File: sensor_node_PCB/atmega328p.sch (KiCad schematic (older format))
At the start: 14 parts, among them SW1 RESET_SWITCH, U5 ATMEGA328P, X2 CSTCE16MOV53-R0

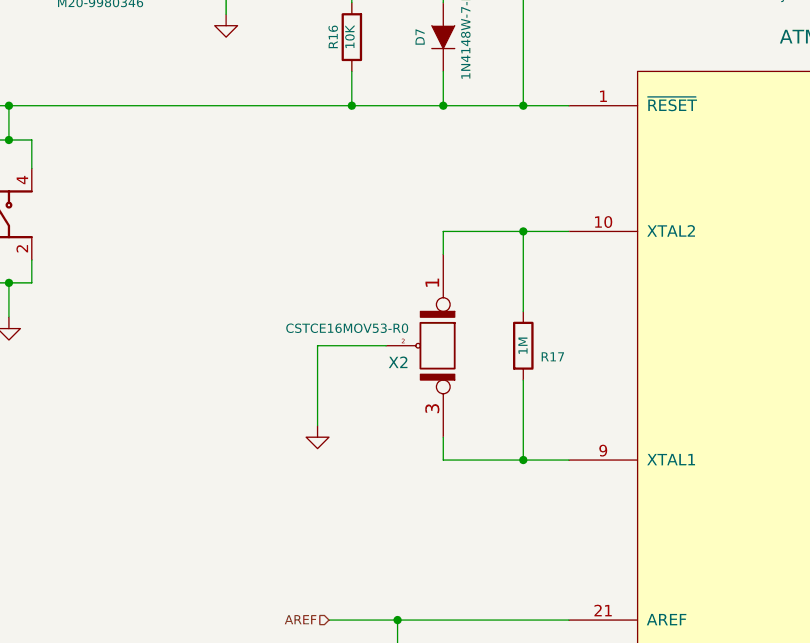
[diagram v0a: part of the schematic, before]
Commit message: routing started 15%
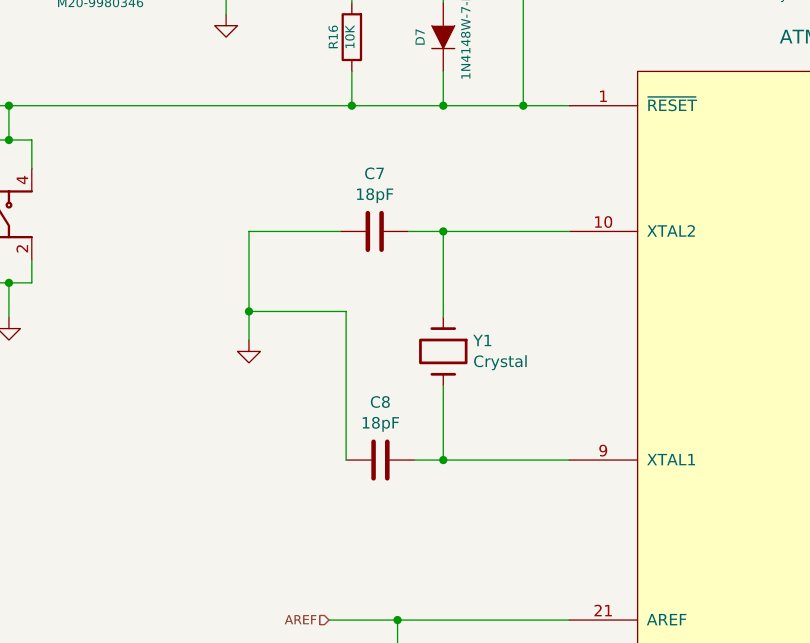
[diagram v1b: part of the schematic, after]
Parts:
- removed R17: 1M, Resistor_SMD:R_0603_1608Metric, symbol Arduino_Uno_R3_From_Scratch-rescue:R
- removed X2: CSTCE16MOV53-R0, symbol Arduino_Uno_R3_From_Scratch-rescue:CERAMIC_RESONATOR
- added C7, C8: 18pF, Capacitor_SMD:C_0603_1608Metric, symbol Arduino_Uno_R3_From_Scratch-rescue:C
- added Y1: Crystal, Crystal:Crystal_SMD_5032-2Pin_5.0x3.2mm, symbol Arduino_Uno_R3_From_Scratch-rescue:Crystal
- D7: footprint (none) -> Diode_SMD:D_SOD-123
- ICSP2: footprint (none) -> Connector_PinHeader_2.54mm:PinHeader_2x03_P2.54mm_Vertical_SMD
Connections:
- net GND: now also C7.2, C8.2
- net at U5.10 (XTAL2): now also C7.1, Y1.1
- net at U5.9 (XTAL1): now also C8.1, Y1.2
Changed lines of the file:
@@
 	1    0    0    -1
 $EndComp
-Wire Wire Line
-	5650 2050 5650 2400
-Connection ~ 5650 2050
-Wire Wire Line
-	5650 2700 5650 3050
-Connection ~ 5650 3050
 Text HLabel 4800 3750 0    40   Input ~ 0
 AREF
@@
 F 0 "ICSP2" H 3800 1100 50  0000 C CNN
 F 1 "M20-9980346" H 3800 650 40  0000 C CNN
-F 2 "" H 3800 850 60  0001 C CNN
+F 2 "Connector_PinHeader_2.54mm:PinHeader_2x03_P2.54mm_Vertical_SMD" H 3800 850 60  0001 C CNN
 F 3 "http://cdn.harwin.com/pdfs/M20-998.pdf" H 3800 850 60  0001 C CNN
 F 4 "6 CONTACT(S), MALE, STRAIGHT TWO PART BOARD CONNECTOR" H 3800 850 60  0001 C CNN "Characteristics"
@@
 F 0 "D7" H 5300 1300 40  0000 C CNN
 F 1 "1N4148W-7-F" H 5300 1100 40  0000 C CNN
-F 2 "" H 5300 1200 60  0001 C CNN
+F 2 "Diode_SMD:D_SOD-123" H 5300 1200 60  0001 C CNN
 F 3 "http://www.diodes.com/_files/datasheets/ds30086.pdf" H 5300 1200 60  0001 C CNN
 F 4 "DIODE GEN PURP 100V 300MA SOD123" H 5300 1200 60  0001 C CNN "Characteristics"
@@
 	0    -1   -1   0
 $EndComp
-$Comp
-L Arduino_Uno_R3_From_Scratch-rescue:CERAMIC_RESONATOR X2
-U 1 1 5614A1DB
-P 5250 2550
-F 0 "X2" V 5325 2450 50  0000 R CNN
-F 1 "CSTCE16MOV53-R0" V 5175 2450 40  0000 R CNN
-F 2 "" H 5250 2550 60  0001 C CNN
-F 3 "http://www.murata.com/~/media/webrenewal/support/library/catalog/products/timingdevice/ceralock/p16e.ashx" H 5250 2550 60  0001 C CNN
-F 4 "CER RESONATOR 16.0MHZ SMD" H 5250 2550 60  0001 C CNN "Characteristics"
-F 5 "ATMEGA328P Oscillator" H 5250 2550 60  0001 C CNN "Description"
-F 6 "Murata" H 5250 2550 60  0001 C CNN "MFN"
-F 7 "CSTCE16M0V53-R0" H 5250 2550 60  0001 C CNN "MFP"
-F 8 "SMD" H 5250 2550 60  0001 C CNN "Package ID"
-F 9 "ANY" H 5250 2550 60  0001 C CNN "Source"
-F 10 "Y" H 5250 2550 60  0001 C CNN "Critical"
-F 11 "328P_Sub" H 5250 2550 60  0001 C CNN "Subsystem"
-F 12 "~" H 5250 2550 60  0001 C CNN "Notes"
-	1    5250 2550
-	0    1    1    0
-$EndComp
-Wire Wire Line
-	5300 2050 5650 2050
-Wire Wire Line
-	5300 2050 5300 2150
-Wire Wire Line
-	5300 2950 5300 3050
-Wire Wire Line
-	5300 3050 5650 3050
-Wire Wire Line
-	5050 2550 4750 2550
-Wire Wire Line
-	4750 2550 4750 2900
 Text Notes 6150 1050 0    40   ~ 0
 Atmel Appnote: AVR042 - AVR Hardware Design Considerations\nhttp://www.atmel.com/Images/Atmel-2521-AVR-Hardware-Design-Considerations_ApplicationNote_AVR042.pdf\n\nRefer to this for PCB layout information
@@
 	0    -1   -1   0
 $EndComp
-$Comp
-L Arduino_Uno_R3_From_Scratch-rescue:R R17
-U 1 1 5615BCD3
-P 5650 2550
-F 0 "R17" H 5725 2500 40  0000 L CNN
-F 1 "1M" V 5650 2550 40  0000 C CNN
-F 2 "Resistor_SMD:R_0603_1608Metric" V 5580 2550 30  0001 C CNN
-F 3 "http://www.vishay.com/docs/20035/dcrcwe3.pdf" H 5650 2550 30  0001 C CNN
-F 4 "RES SMD 1M OHM 1% 1/8W 0805" H 5650 2550 60  0001 C CNN "Characteristics"
-F 5 "ATMEGA328P Xtal 1M Feedback Resistor" H 5650 2550 60  0001 C CNN "Description"
-F 6 "Vishay" H 5650 2550 60  0001 C CNN "MFN"
-F 7 "CRCW08051M00FKEA" H 5650 2550 60  0001 C CNN "MFP"
-F 8 "SMD_0805" H 5650 2550 60  0001 C CNN "Package ID"
-F 9 "ANY" H 5650 2550 60  0001 C CNN "Source"
-F 10 "N" H 5650 2550 60  0001 C CNN "Critical"
-F 11 "328P_Sub" H 5650 2550 60  0001 C CNN "Subsystem"
-F 12 "~" H 5650 2550 60  0001 C CNN "Notes"
-	1    5650 2550
-	1    0    0    -1
-$EndComp
 Wire Wire Line
 	3500 1650 3500 1775
@@
 L Arduino_Uno_R3_From_Scratch-rescue:GND #PWR044
 U 1 1 56207870
-P 4750 2900
-F 0 "#PWR044" H 4750 2900 30  0001 C CNN
-F 1 "GND" H 4750 2830 30  0001 C CNN
-F 2 "~" H 4750 2900 60  0000 C CNN
-F 3 "~" H 4750 2900 60  0000 C CNN
-F 4 "ANY" H 4750 2900 60  0001 C CNN "Source"
-F 5 "N" H 4750 2900 60  0001 C CNN "Critical"
-F 6 "~" H 4750 2900 60  0001 C CNN "Notes"
-	1    4750 2900
+P 4450 2525
+F 0 "#PWR044" H 4450 2525 30  0001 C CNN
+F 1 "GND" H 4450 2455 30  0001 C CNN
+F 2 "~" H 4450 2525 60  0000 C CNN
+F 3 "~" H 4450 2525 60  0000 C CNN
+F 4 "ANY" H 4450 2525 60  0001 C CNN "Source"
+F 5 "N" H 4450 2525 60  0001 C CNN "Critical"
+F 6 "~" H 4450 2525 60  0001 C CNN "Notes"
+	1    4450 2525
 	1    0    0    -1
 $EndComp
@@
 $EndComp
 Wire Wire Line
-	5650 2050 5850 2050
-Wire Wire Line
-	5650 3050 5850 3050
-Wire Wire Line
 	5600 4500 5600 4700
 Wire Wire Line
@@
 Wire Wire Line
 	5650 1500 5850 1500
+Wire Wire Line
+	5300 3050 5850 3050
+Wire Wire Line
+	5300 2050 5850 2050
+$Comp
+L Arduino_Uno_R3_From_Scratch-rescue:Crystal Y1
+U 1 1 5F569D4C
+P 5300 2575
+F 0 "Y1" V 5254 2706 50  0000 L CNN
+F 1 "Crystal" V 5345 2706 50  0000 L CNN
+F 2 "Crystal:Crystal_SMD_5032-2Pin_5.0x3.2mm" H 5300 2575 60  0001 C CNN
+F 3 "" H 5300 2575 60  0000 C CNN
+	1    5300 2575
+	0    1    1    0
+$EndComp
+Wire Wire Line
+	5300 2050 5300 2425
+Wire Wire Line
+	5300 2725 5300 3050
+$Comp
+L Arduino_Uno_R3_From_Scratch-rescue:C C7
+U 1 1 5F570541
+P 5000 2050
+F 0 "C7" V 4748 2050 50  0000 C CNN
+F 1 "18pF" V 4839 2050 50  0000 C CNN
+F 2 "Capacitor_SMD:C_0603_1608Metric" H 5038 1900 30  0001 C CNN
+F 3 "" H 5000 2050 60  0000 C CNN
+	1    5000 2050
+	0    1    1    0
+$EndComp
+$Comp
+L Arduino_Uno_R3_From_Scratch-rescue:C C8
+U 1 1 5F570D63
+P 5025 3050
+F 0 "C8" V 4773 3050 50  0000 C CNN
+F 1 "18pF" V 4864 3050 50  0000 C CNN
+F 2 "Capacitor_SMD:C_0603_1608Metric" H 5063 2900 30  0001 C CNN
+F 3 "" H 5025 3050 60  0000 C CNN
+	1    5025 3050
+	0    1    1    0
+$EndComp
+Wire Wire Line
+	5150 2050 5300 2050
+Connection ~ 5300 2050
+Wire Wire Line
+	5175 3050 5300 3050
+Connection ~ 5300 3050
+Wire Wire Line
+	4850 2050 4450 2050
+Wire Wire Line
+	4450 2050 4450 2400
+Wire Wire Line
+	4875 3050 4875 2400
+Wire Wire Line
+	4875 2400 4450 2400
+Connection ~ 4450 2400
+Wire Wire Line
+	4450 2400 4450 2525
 $EndSCHEMATC
